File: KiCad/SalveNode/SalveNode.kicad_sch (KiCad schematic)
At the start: 2 parts, among them IC1 TMP75AQDGKRQ1

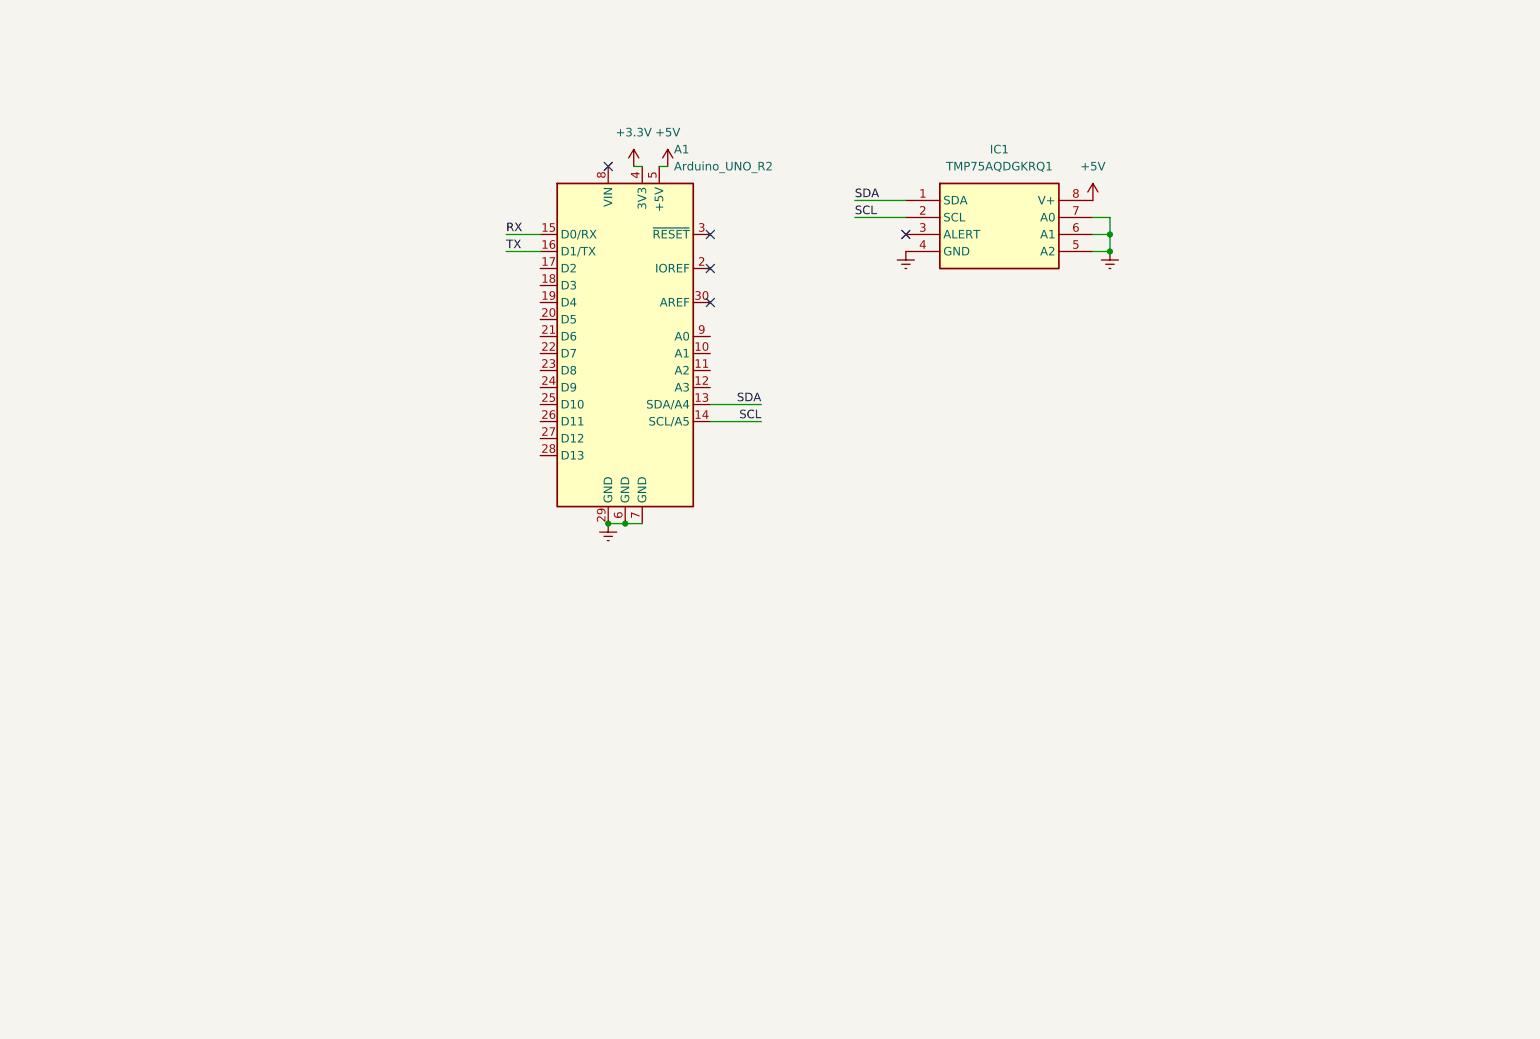
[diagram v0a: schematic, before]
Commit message: tarjeta externa añadido
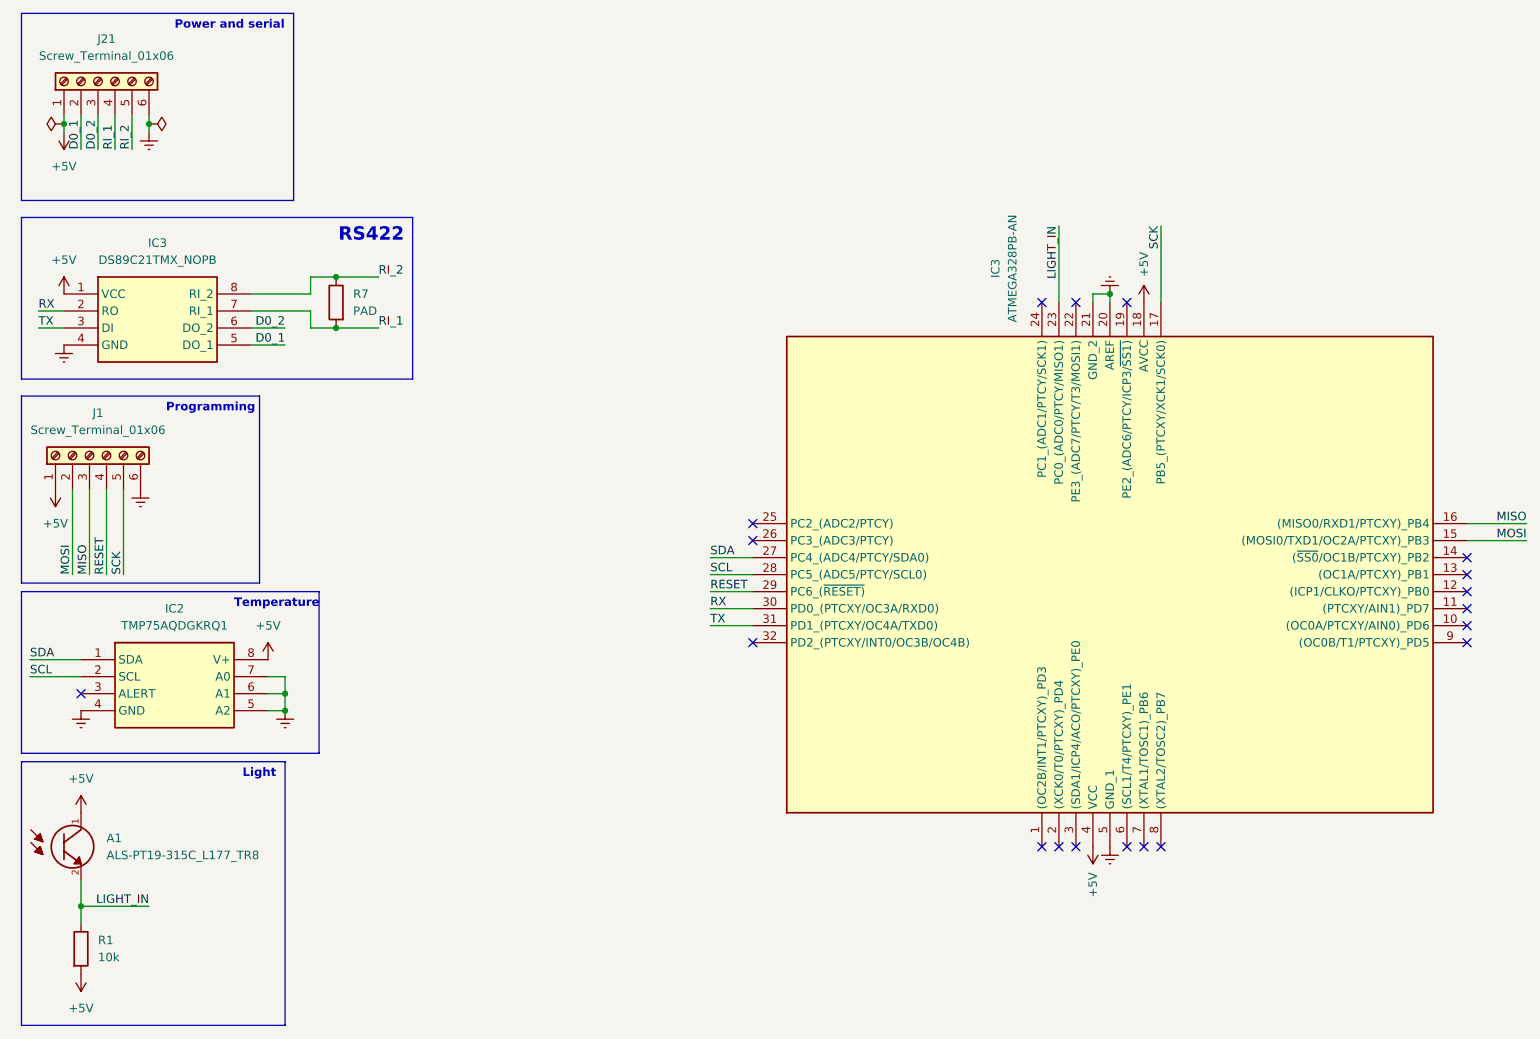
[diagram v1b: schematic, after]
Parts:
- removed A1: Arduino_UNO_R2, Module:Arduino_UNO_R2, symbol MCU_Module:Arduino_UNO_R2
- added A1: ALS-PT19-315C_L177_TR8, ALS-PT19-315C_L177_TR8:XDCR_ALS-PT19-315C_L177_TR8, symbol ALS-PT19-315C_L177_TR8:ALS-PT19-315C_L177_TR8
- added IC3: ATMEGA328PB-AN, QFP80P900X900X120-32N, symbol SamacSys_Parts:ATMEGA328PB-AN
- added IC3: DS89C21TMX_NOPB, SOIC127P600X175-8N, symbol SamacSys_Parts:DS89C21TMX_NOPB
- added J1, J21: Screw_Terminal_01x06, symbol Connector:Screw_Terminal_01x06
- added R1: 10k, symbol Device:R
- added R7: PAD, Resistor_SMD:R_1206_3216Metric_Pad1.30x1.75mm_HandSolder, symbol Device:R
- renumbered IC1 to IC2
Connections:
- net +5V: now also A1.1, IC3.1 (VCC), IC3.18 (AVCC), IC3.4 (VCC), J1.1 (Pin_1), J21.1 (Pin_1), R1.2
- net Earth: now also IC3.20 (AREF), IC3.21 (GND_2), IC3.4 (GND), IC3.5 (GND_1), J1.6 (Pin_6), J21.6 (Pin_6)
- net RX: now also IC3.2 (RO), IC3.30 (PD0_(PTCXY/OC3A/RXD0))
- net SCL: now also IC3.28 (PC5_(ADC5/PTCY/SCL0))
- net SDA: now also IC3.27 (PC4_(ADC4/PTCY/SDA0))
- net TX: now also IC3.3 (DI), IC3.31 (PD1_(PTCXY/OC4A/TXD0))
- new net D0_1: IC3.5 (DO_1), J21.2 (Pin_2)
- new net D0_2: IC3.6 (DO_2), J21.3 (Pin_3)
- new net LIGHT_IN: A1.2, IC3.23 (PC0_(ADC0/PTCY/MISO1)), R1.1
- new net MISO: IC3.16 ((MISO0/RXD1/PTCXY)_PB4), J1.3 (Pin_3)
- new net MOSI: IC3.15 ((MOSI0/TXD1/OC2A/PTCXY)_PB3), J1.2 (Pin_2)
- new net RESET: IC3.29 (PC6_(~{RESET)}), J1.4 (Pin_4)
- new net RI_1: IC3.7 (RI_1), J21.4 (Pin_4), R7.2
- new net RI_2: IC3.8 (RI_2), J21.5 (Pin_5), R7.1
- new net SCK: IC3.17 (PB5_(PTCXY/XCK1/SCK0)), J1.5 (Pin_5)
- no-connect marks 5 -> 19
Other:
- note added: "Light"
- note added: "Power and serial"
- note added: "Programming"
- note added: "RS422"
- note added: "Temperature"
- moved on the sheet: IC2
